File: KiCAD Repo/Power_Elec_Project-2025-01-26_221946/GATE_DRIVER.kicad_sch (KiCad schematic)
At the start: 0 parts

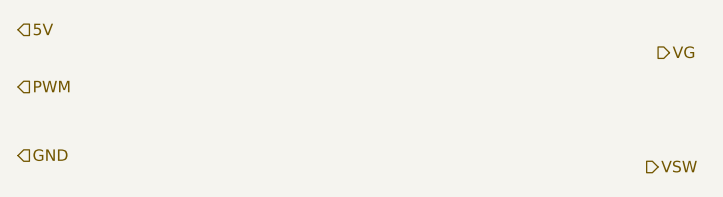
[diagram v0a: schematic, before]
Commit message: lpf design
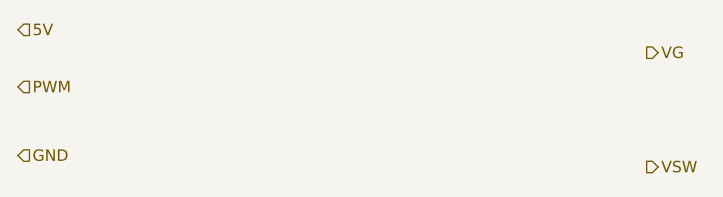
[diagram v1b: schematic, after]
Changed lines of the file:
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@@
 	(hierarchical_label "VG"
 		(shape output)
-		(at 191.77 29.21 0)
+		(at 190.5 29.21 0)
 		(effects
 			(font
